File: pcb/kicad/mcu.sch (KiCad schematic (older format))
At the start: 2 parts, among them U11 LPC1754

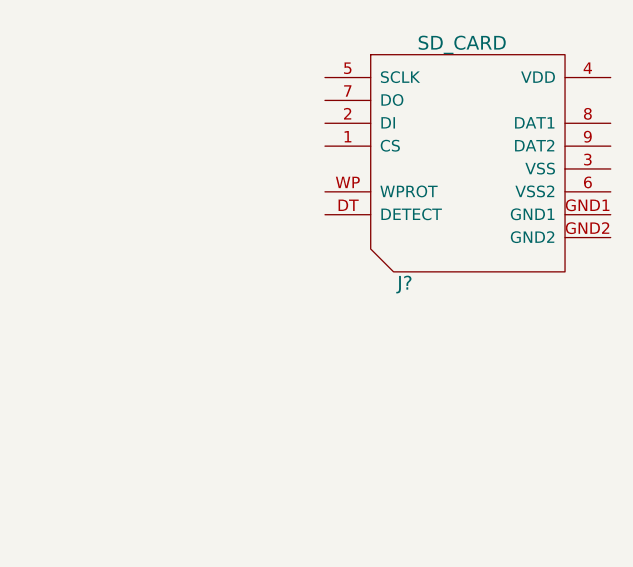
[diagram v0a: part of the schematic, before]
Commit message: kicad wip
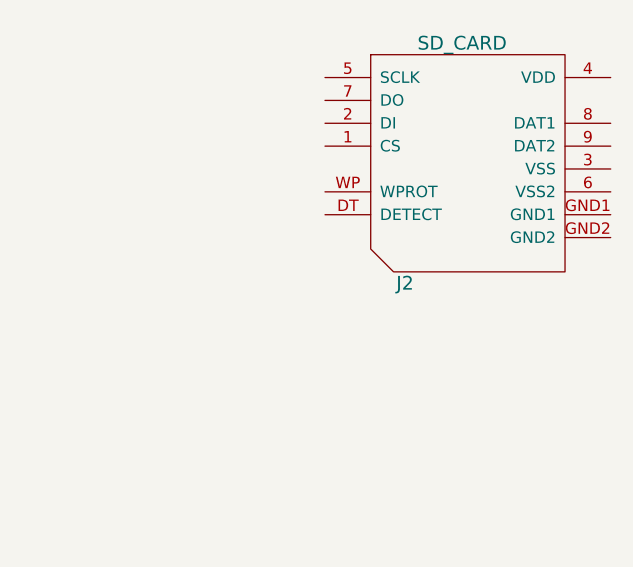
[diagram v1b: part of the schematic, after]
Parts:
- gave numbers to parts that had none: 1
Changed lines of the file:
@@
-EESchema Schematic File Version 2  date Wed 24 Mar 2010 11:33:24 PM CET
-LIBS:sd2snes-cache
+EESchema Schematic File Version 2  date Sat 27 Mar 2010 11:02:39 PM CET
 LIBS:power
 LIBS:device
@@
 LIBS:mt45w8mw16
 LIBS:cs4344
+LIBS:sd2snes-cache
 EELAYER 24  0
 EELAYER END
 $Descr A4 11700 8267
 Sheet 3 6
-Title ""
-Date "9 feb 2010"
-Rev ""
-Comp ""
+Title "sd2snes Mark II"
+Date "27 mar 2010"
+Rev "A"
+Comp "Maximilian Rehkopf"
 Comment1 ""
 Comment2 ""
@@
 $EndDescr
 $Comp
-L SD_CARD J?
+L SD_CARD J2
 U 1 1 4BAA6A9C
 P 8650 2500
-F 0 "J?" H 8400 1950 60  0000 C CNN
+F 0 "J2" H 8400 1950 60  0000 C CNN
 F 1 "SD_CARD" H 8650 3000 60  0000 C CNN
 	1    8650 2500

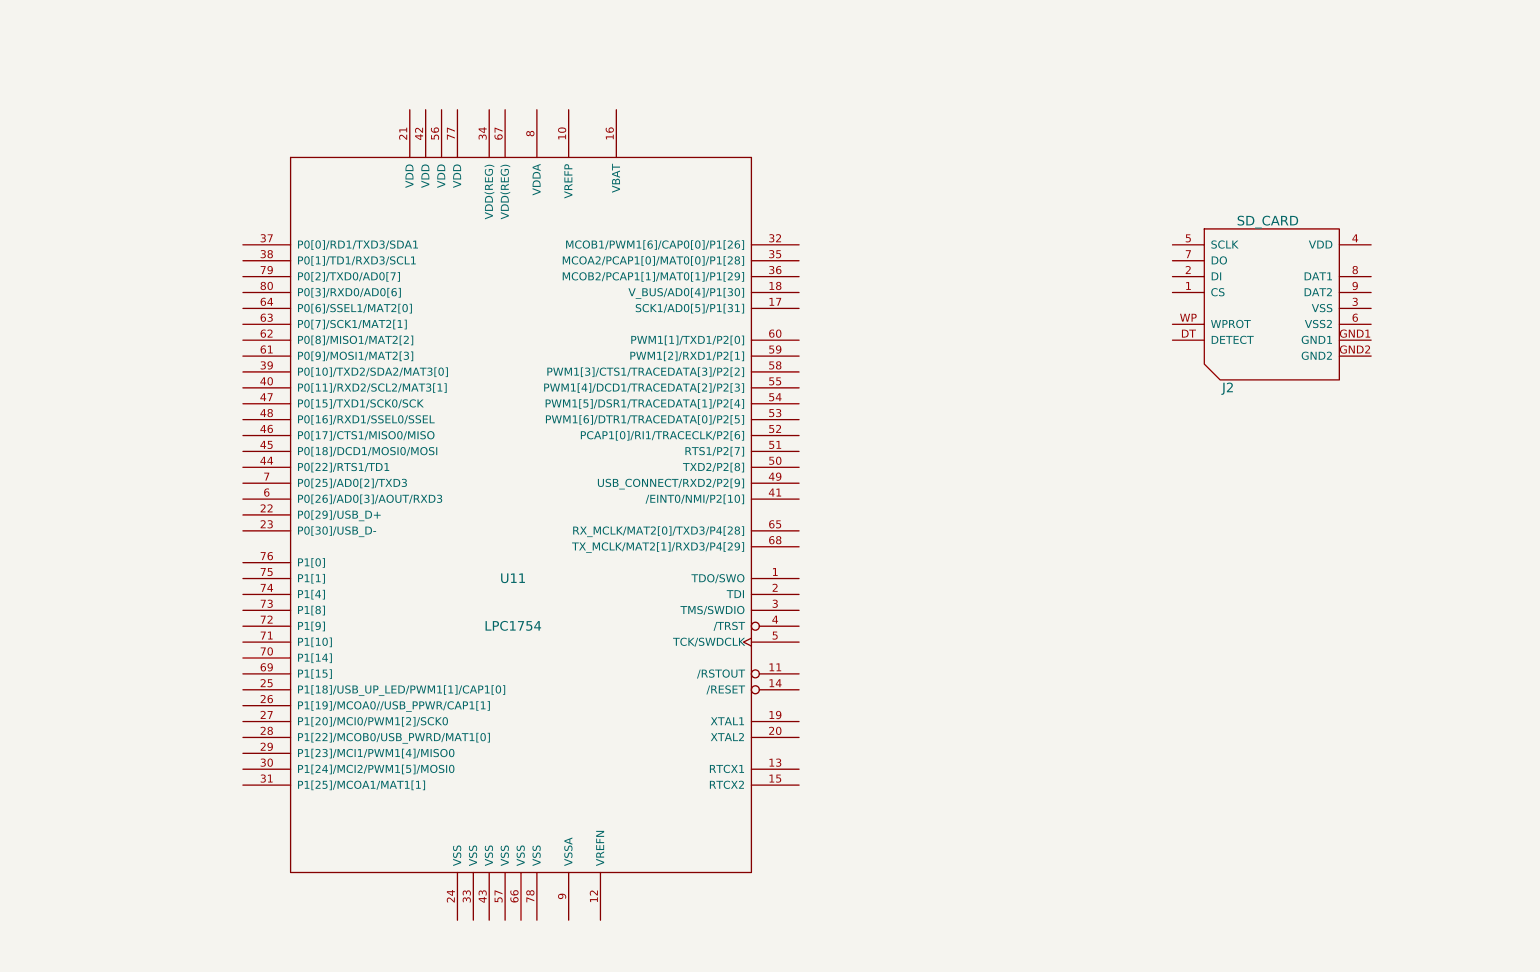
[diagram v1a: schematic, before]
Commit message: Schematics+PCB WIP
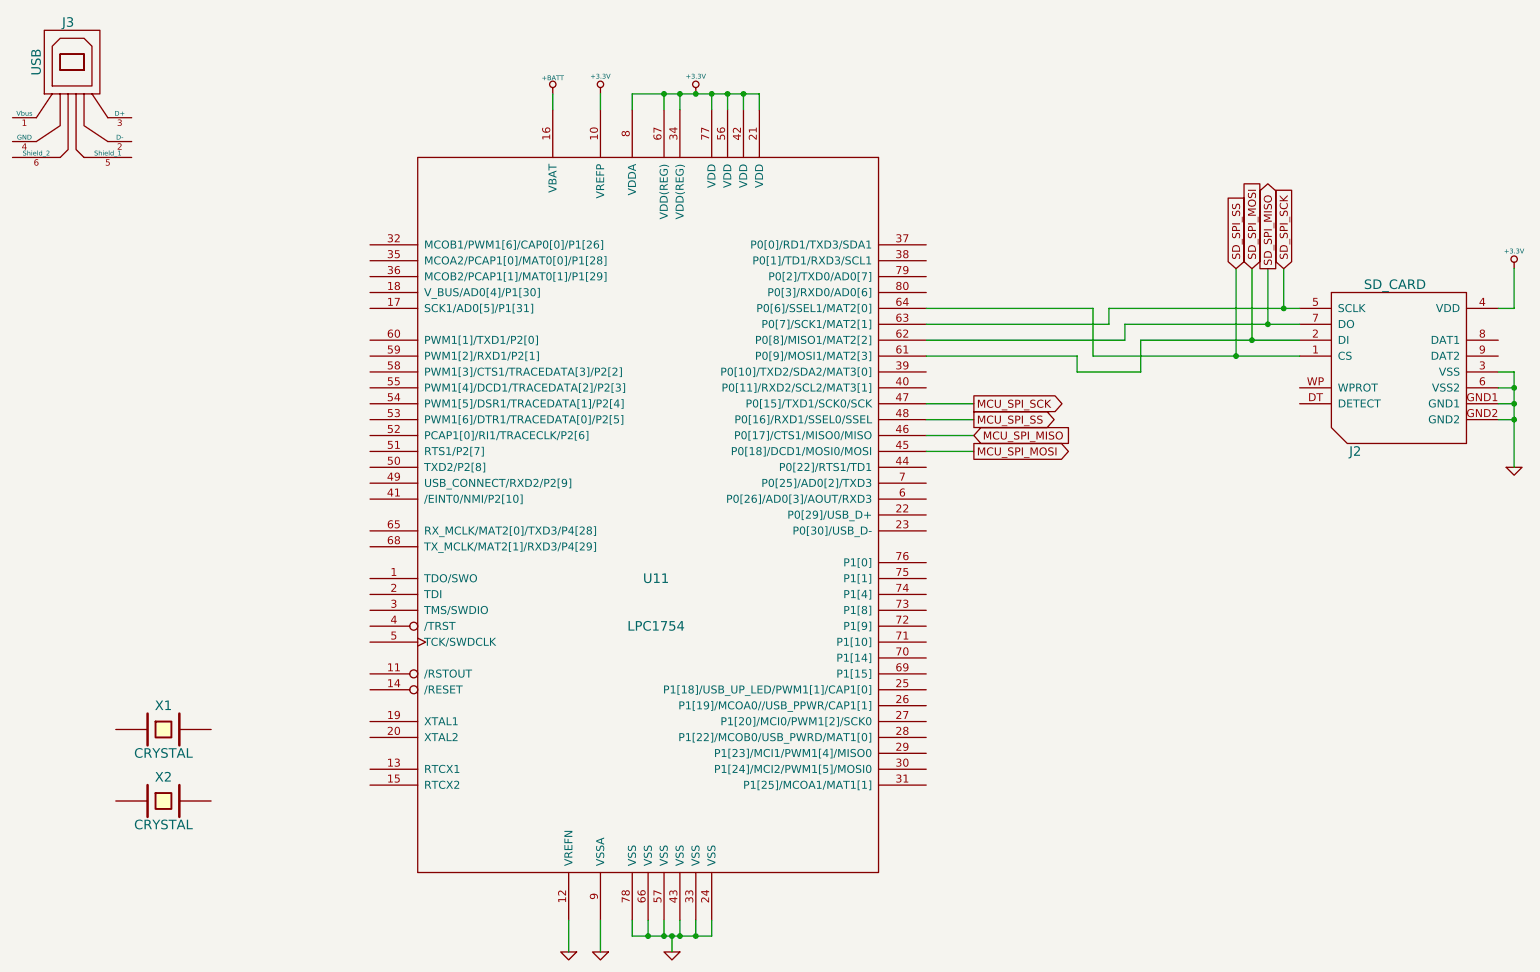
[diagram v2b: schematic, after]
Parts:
- added J3: USB, symbol USB
- added X1, X2: CRYSTAL, symbol CRYSTAL
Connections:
- net +3.3V: now reaches U11.10 (VREFP)
- net +3.3V: now also J2.4 (VDD), U11.21 (VDD), U11.34 (VDD(REG)), U11.42 (VDD), U11.56 (VDD), U11.67 (VDD(REG)), U11.77 (VDD), U11.8 (VDDA)
- net GND: now reaches U11.12 (VREFN)
- net GND: now also J2.3 (VSS), J2.6 (VSS2), J2.GND1, J2.GND2, U11.24 (VSS), U11.33 (VSS), U11.43 (VSS), U11.57 (VSS), U11.66 (VSS), U11.78 (VSS), U11.9 (VSSA)
- net +BATT: now reaches U11.16 (VBAT)
- net MCU_SPI_MOSI: now reaches U11.45 (P0[18]/DCD1/MOSI0/MOSI)
- net MCU_SPI_MISO: now reaches U11.46 (P0[17]/CTS1/MISO0/MISO)
- net MCU_SPI_SCK: now reaches U11.47 (P0[15]/TXD1/SCK0/SCK)
- net MCU_SPI_SS: now reaches U11.48 (P0[16]/RXD1/SSEL0/SSEL)
- net SD_SPI_MOSI: now reaches U11.61 (P0[9]/MOSI1/MAT2[3])
- net SD_SPI_MOSI: now also J2.2 (DI)
- net SD_SPI_MISO: now reaches U11.62 (P0[8]/MISO1/MAT2[2])
- net SD_SPI_MISO: now also J2.7 (DO)
- net SD_SPI_SCK: now reaches U11.63 (P0[7]/SCK1/MAT2[1])
- net SD_SPI_SCK: now also J2.5 (SCLK)
- net SD_SPI_SS: now reaches U11.64 (P0[6]/SSEL1/MAT2[0])
- net SD_SPI_SS: now also J2.1 (CS)
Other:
- moved on the sheet: J2, U11
